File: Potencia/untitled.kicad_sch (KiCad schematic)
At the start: 13 parts, among them U3.3 LM2596S-3.3, U5 LM2596S-5

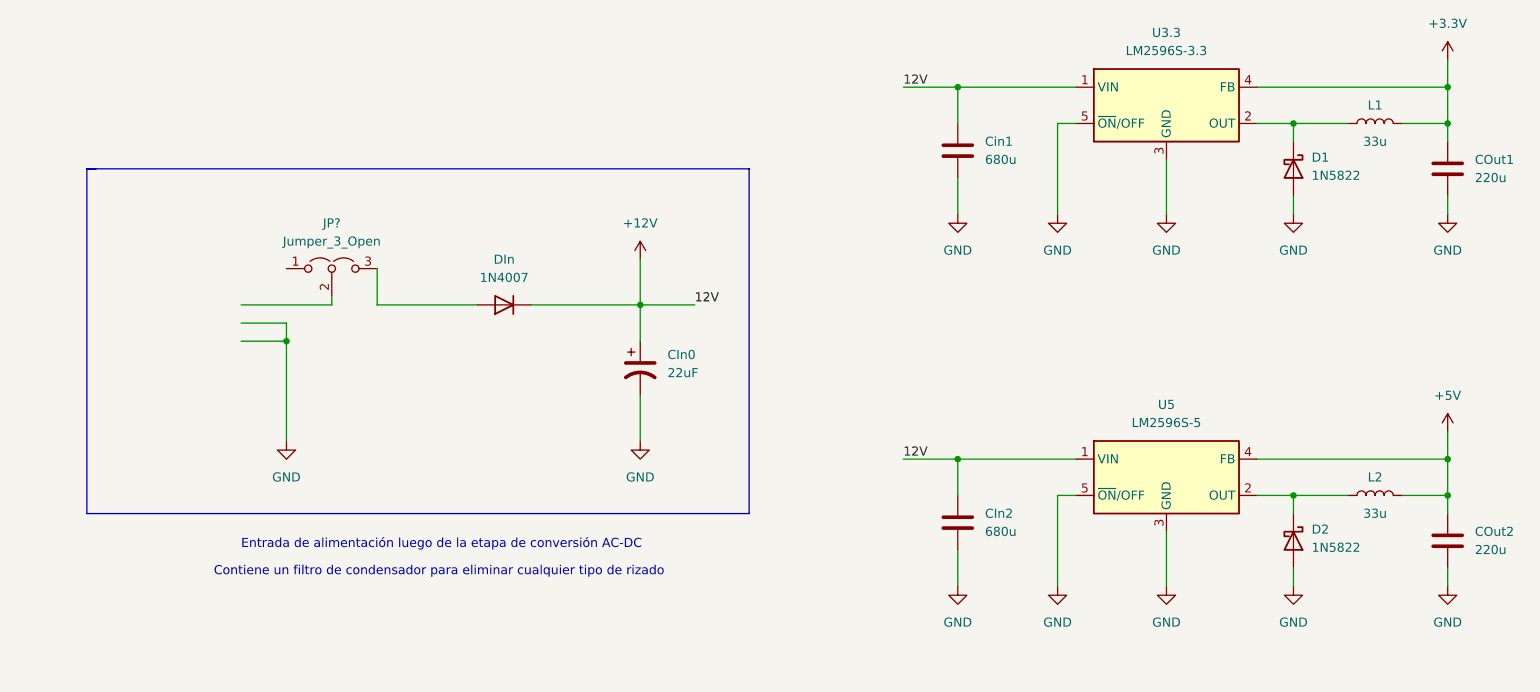
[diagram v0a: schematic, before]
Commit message: Bloques_CircuitoPotencia_ControlPilot
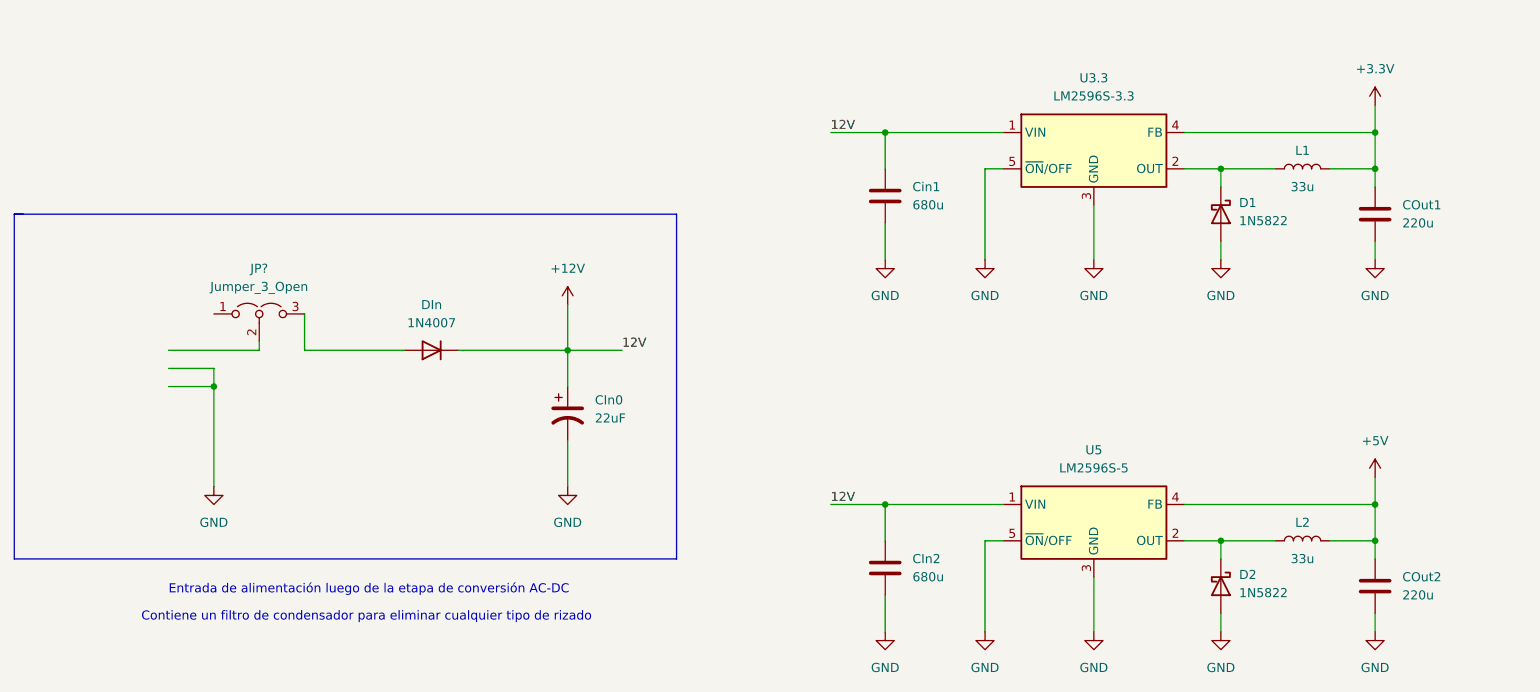
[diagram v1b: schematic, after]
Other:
- moved on the sheet: CIn0, CIn2, COut1, COut2, Cin1, D1, D2, DIn, JP?, L1, L2, U3.3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
